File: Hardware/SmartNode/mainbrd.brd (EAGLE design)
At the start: 50.5 x 24.1 mm, 42 parts, among them U1 NRF51822-QFAA, U2 CC3000, X1 87438-06, Y1 16MHz, Y2 32.768kHz

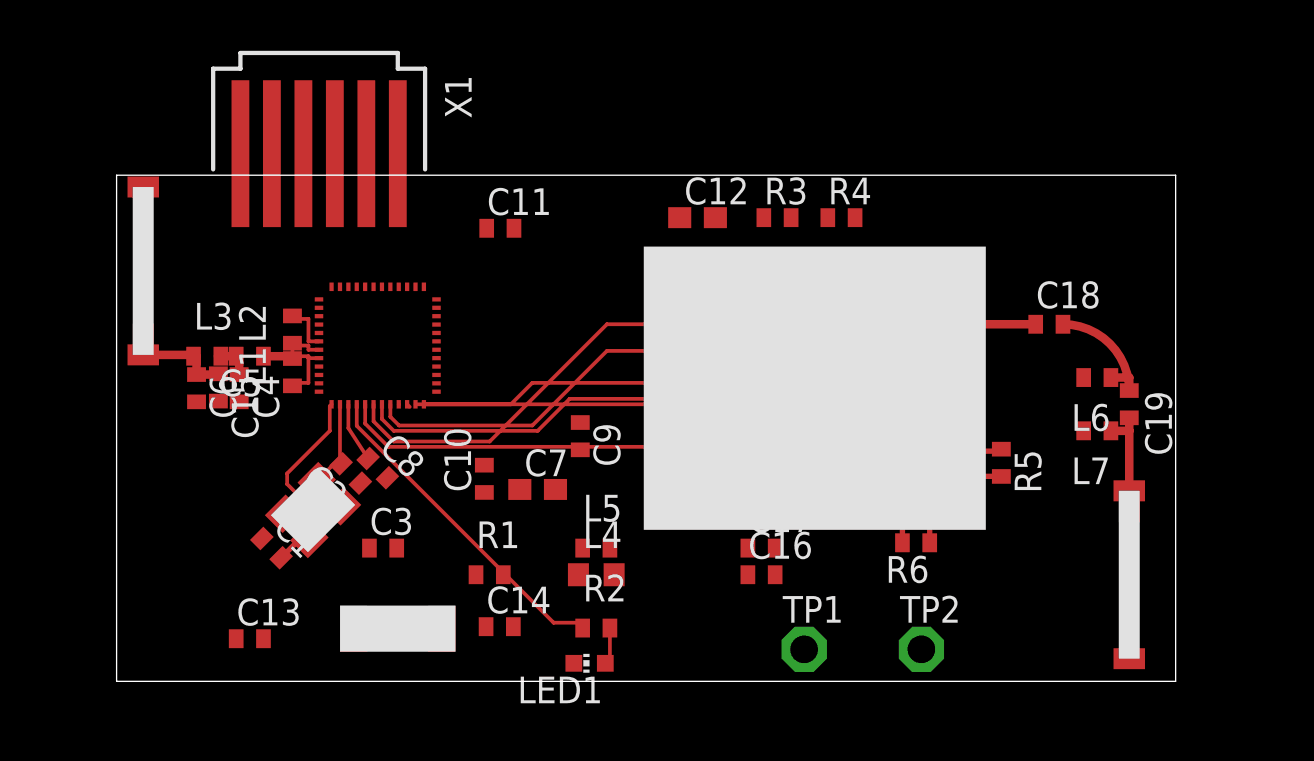
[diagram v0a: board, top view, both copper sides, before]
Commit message: Updated Hardware Files
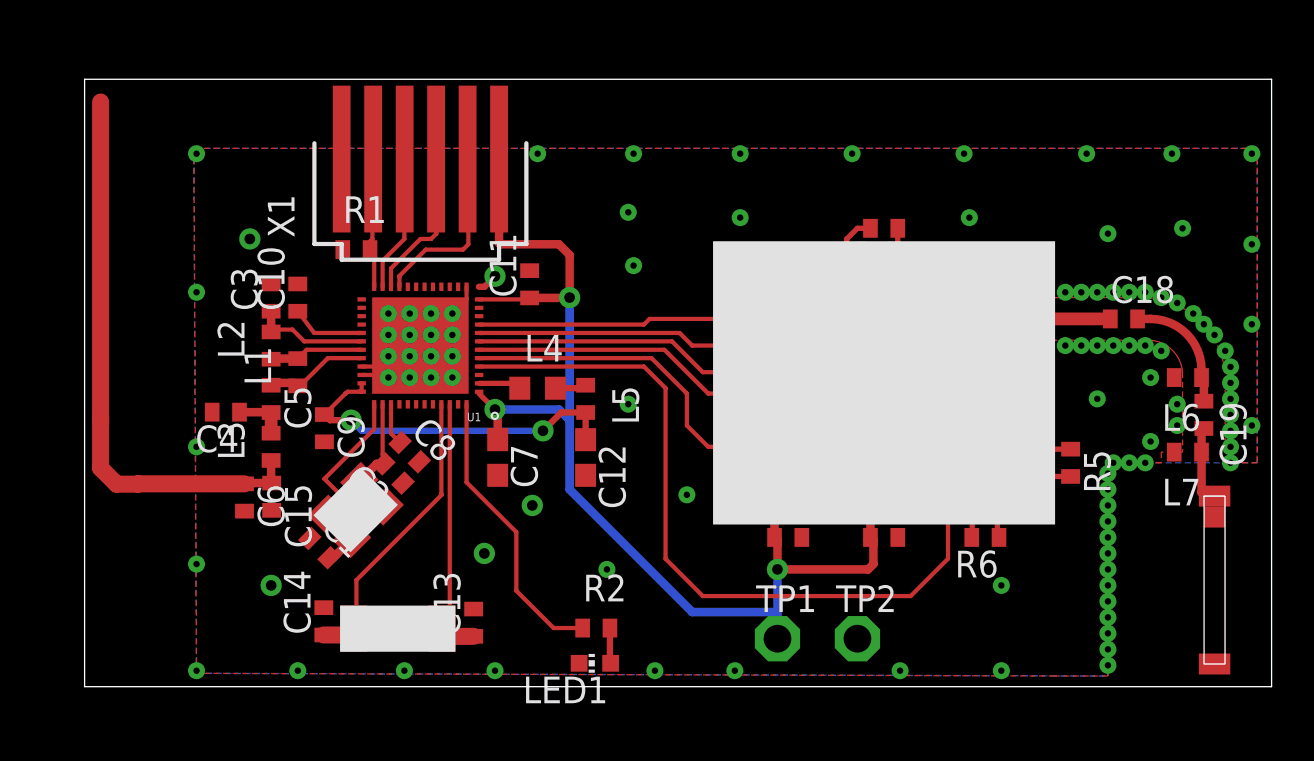
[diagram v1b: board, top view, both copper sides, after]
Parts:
- removed R3: NL, rcl:R0402
- U$2: value AT8010 -> PCB_ANT; device SmartNodeLib:AT8010 -> SmartNodeLib:PCB_ANT
- moved R1 16.7 mm to (29.2, 33.3)
- moved C3 13.1 mm to (25.1, 31.0), turned to 90 degrees
- moved C12 12.6 mm to (40.1, 23.4), turned to 270 degrees
- moved C10 12.4 mm to (26.4, 31.0)
- moved C9 12.2 mm to (27.7, 24.8)
- moved C13 10.7 mm to (34.8, 15.5), turned to 90 degrees
- moved L4 9.32 mm to (37.8, 26.7)
- moved C14 8.39 mm to (27.7, 15.6), turned to 90 degrees
- moved L5 7.13 mm to (40.1, 26.2), turned to 270 degrees
- moved C17 5.86 mm to (54.4, 19.6)
- moved C15 5.79 mm to (25.2, 21.5)
- moved C6 5.69 mm to (23.9, 21.5)
- moved L3 5.29 mm to (25.1, 23.9), turned to 90 degrees
- moved X1 4.83 mm to (32.3, 37.6), turned to 90 degrees
- moved L7 4.44 mm to (68.8, 23.6)
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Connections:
- removed net N$11: C15.1, C6.1, L3.1, U$2.FP
- new net ANT: C15.1, C6.1, L3.1, U$2.P$1
- net GND: no longer R3.1
- net N$16: now also U1.48; no longer U1.40
- net N$19: no longer R3.2
- net SPI_CLK: now also U1.5; no longer U1.41
- net SPI_CS: now also U1.9; no longer U1.42
- net SPI_IRQ: now also U1.7; no longer U1.47
- net SPI_MISO: now also U1.8; no longer U1.44
- net SPI_MOSI: now also U1.6; no longer U1.43
- net UART_RX: now also U1.21, X1.5; no longer U1.22, X1.4
- net UART_TX: now also U1.22, X1.4; no longer U1.21, X1.5
- net VBAT_SW_EN: now also U1.4; no longer U1.48
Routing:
- net VCC: track 0.00 -> 56.0 mm, vias 0 -> 3
- net AVDD: track 0.00 -> 17.0 mm, vias 0 -> 2
- net N$15: track 0.02 -> 14.0 mm
- net N$14: track 0.18 -> 12.7 mm
- net ANT: track 0.00 -> 12.0 mm
- net VBAT_SW_EN: track 23.7 -> 34.9 mm
- net UART_RX: track 0.00 -> 8.52 mm
- net UART_TX: track 0.00 -> 7.29 mm
- net SWDIO: track 0.00 -> 6.52 mm
- net SWDCLK: track 0.00 -> 6.19 mm
- net GND: track 0.00 -> 5.35 mm, vias 0 -> 113
- net SPI_CS: track 17.3 -> 12.2 mm
- net N$11: track 4.56 -> 0.00 mm
- net N$9: track 0.00 -> 3.56 mm
- net N$8: track 2.48 -> 5.57 mm
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- added copper zone on layer 1, net GND
- added copper zone on layer 16, net GND
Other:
- board size 50.5 x 24.1 mm -> 56.6 x 28.9 mm

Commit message: sync everything up
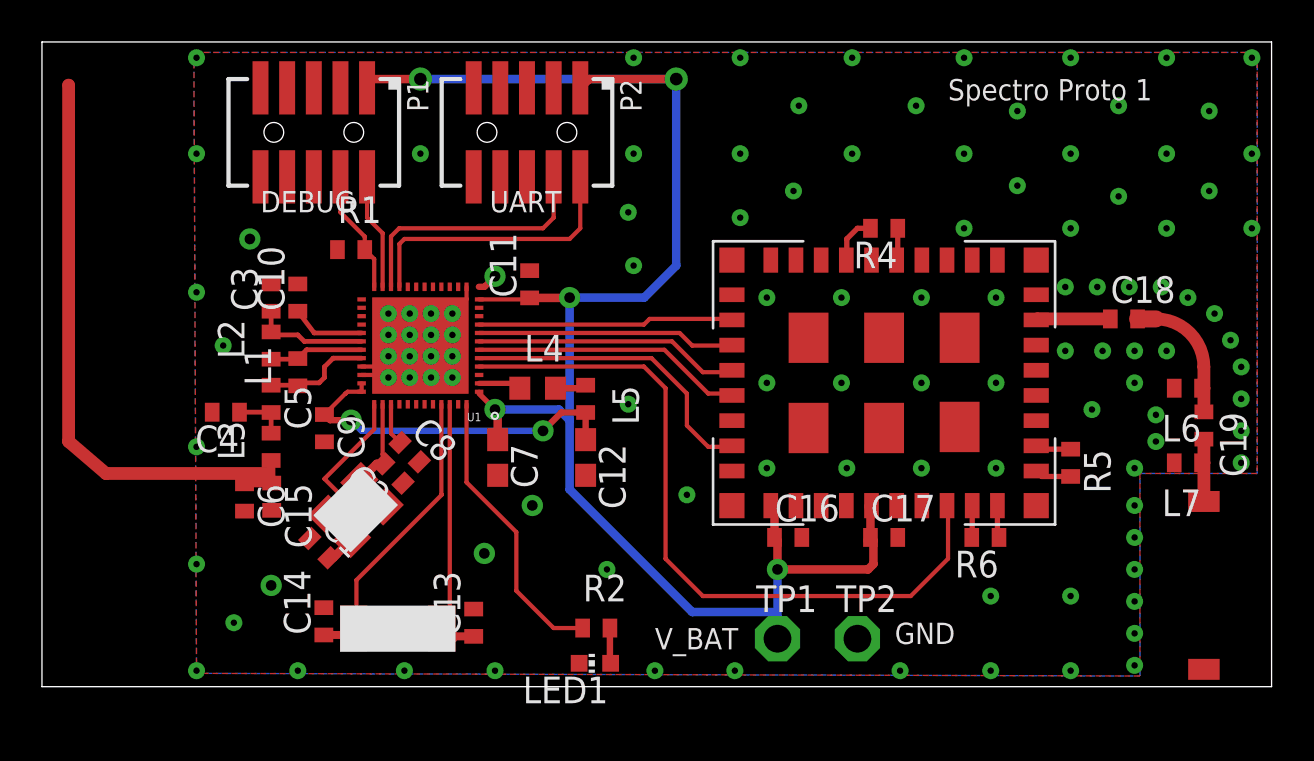
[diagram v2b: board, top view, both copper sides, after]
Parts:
- removed X1: 87438-06, con-molex:87438-06
- added P1, P2: FTSH-105-01-L-DV-K, con-samtec:FTSH-105-01-L-DV-K
- moved U$2 9.02 mm to (15.5, 41.1)
- moved U$1 0.57 mm to (69.6, 17.3)
- moved C19 0.51 mm to (69.6, 24.9)
- moved L6 0.51 mm to (68.8, 26.7)
- moved L7 0.51 mm to (68.8, 23.1)
- moved R1 0.25 mm to (29.0, 33.3)
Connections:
- net GND: now also P1.3, P1.5, P1.9, P2.3, P2.5, P2.9; no longer X1.1
- net SWDCLK: now also P1.4; no longer X1.2
- net SWDIO: now also P1.2; no longer X1.3
- net UART_RX: now also P2.2; no longer X1.5
- net UART_TX: now also P2.4; no longer X1.4
- net VCC: now also P1.1, P2.1; no longer X1.6
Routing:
- net VCC: track 56.0 -> 81.1 mm, vias 3 -> 5
- net ANT: track 12.0 -> 29.9 mm
- net UART_TX: track 7.29 -> 12.5 mm
- net UART_RX: track 8.52 -> 13.4 mm
- net SWDIO: track 6.52 -> 5.55 mm
- net N$24: track 5.57 -> 6.36 mm
- net N$12: track 3.85 -> 3.08 mm
- net GND: vias 113 -> 111
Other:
- board size 56.6 x 28.9 mm -> 58.6 x 30.7 mm
- board text added: "DEBUG"
- board text added: "GND"
- board text added: "Spectro Proto 1"
- board text added: "UART"
- board text added: "V_BAT"
